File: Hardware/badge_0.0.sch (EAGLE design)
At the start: 48 parts, among them CON1 PH_2, IC1 CP2102, J3 2X6 FEMALE, SW1 MK12C02, SW2 MK12C02, U1 SMBT2222A, U2 SMBT2222A, U4 MCP73832T-2DCI/OT

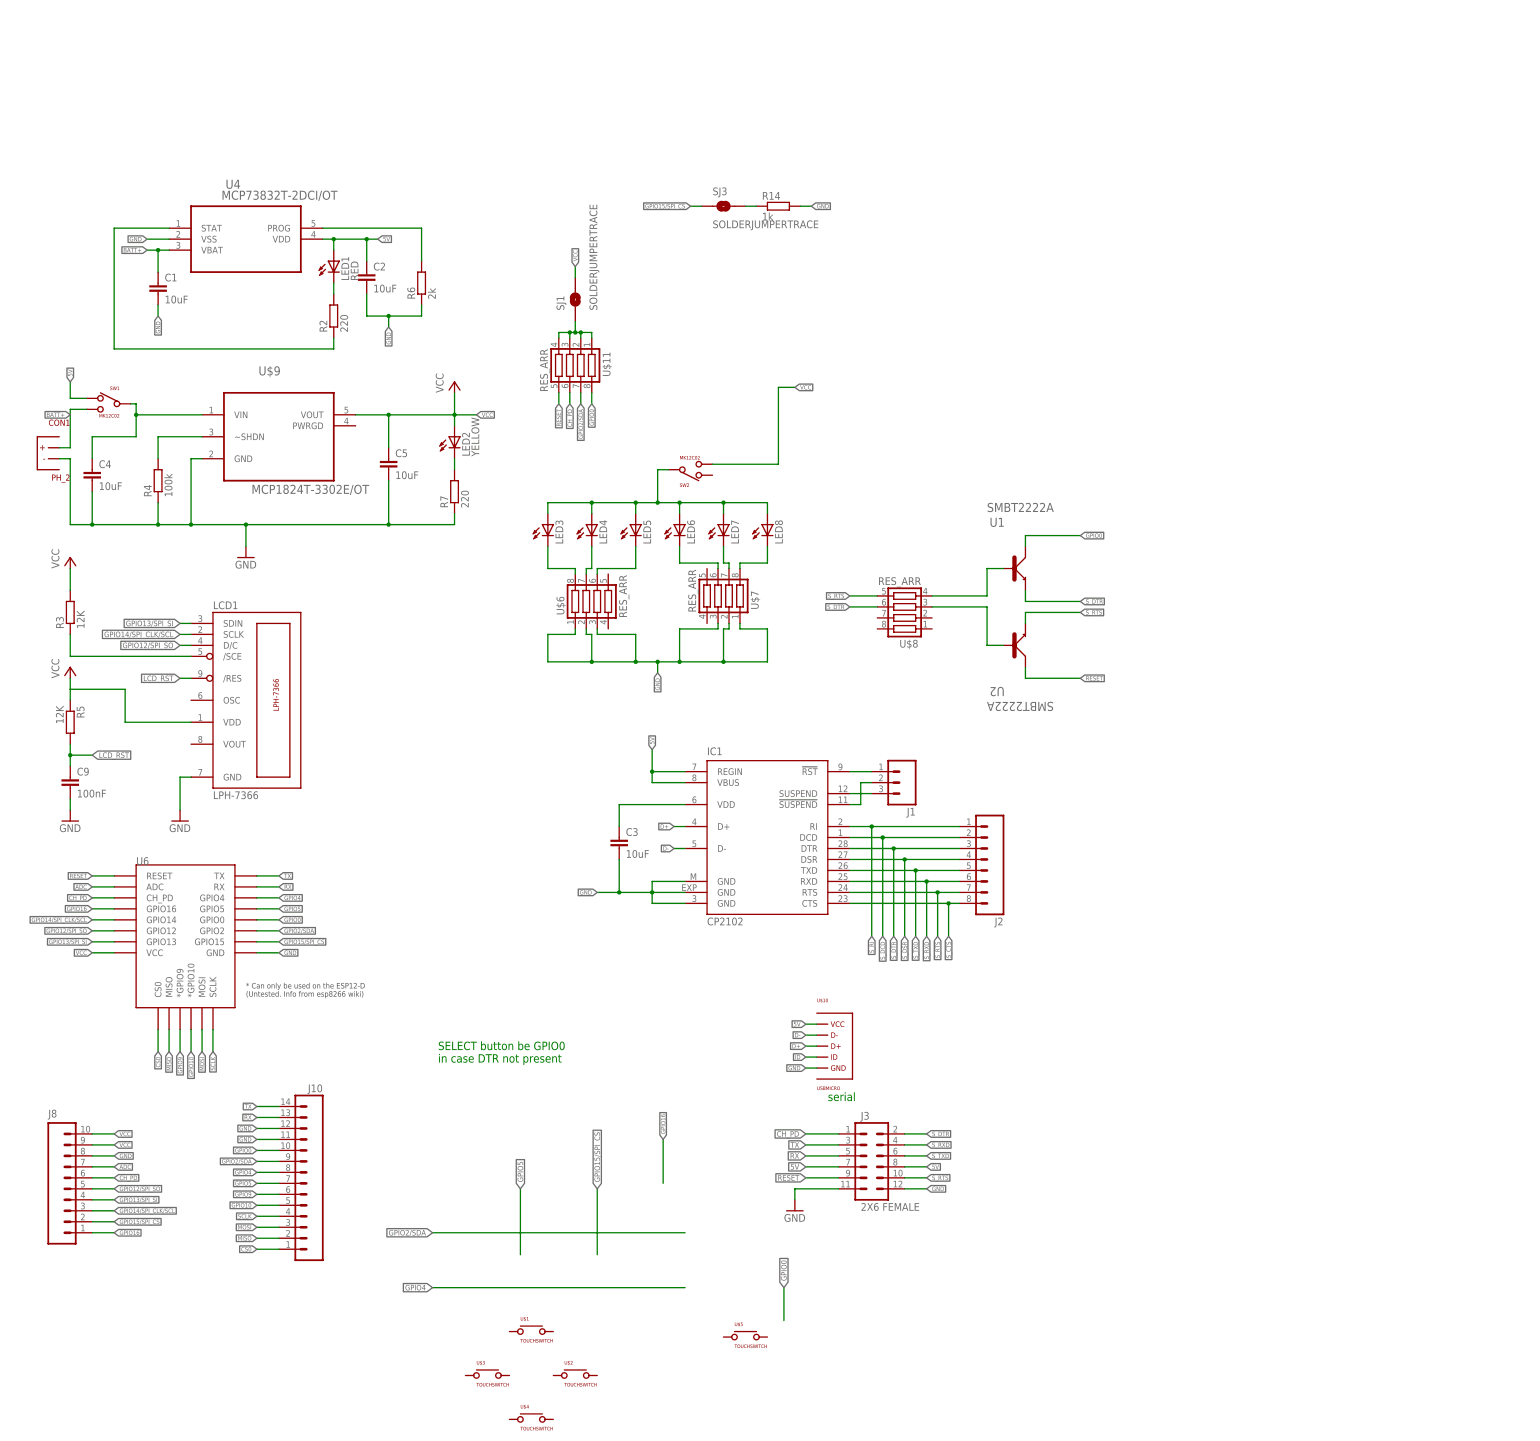
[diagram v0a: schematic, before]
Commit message: Preliminary Neander v0.0
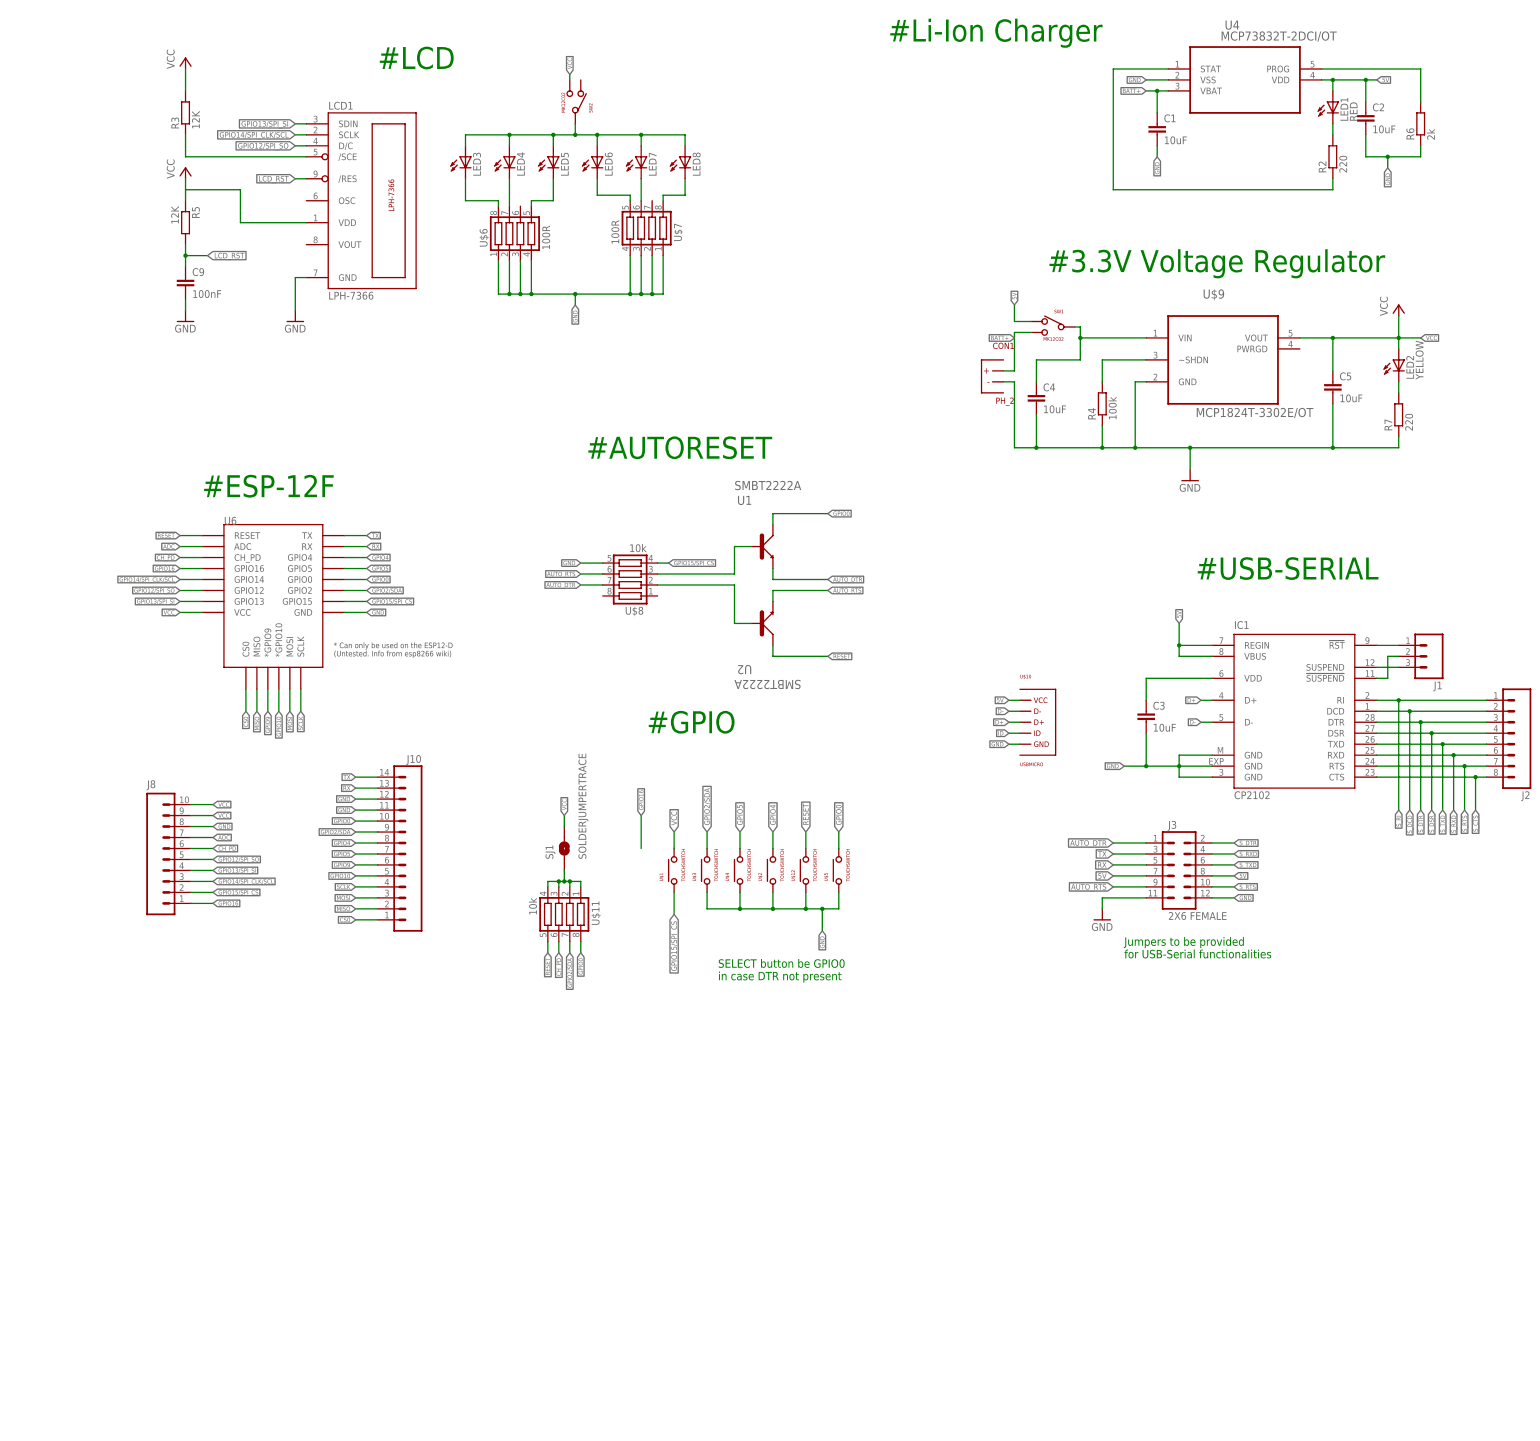
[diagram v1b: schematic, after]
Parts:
- removed R14: 1k, resistor:R-EU_R0603W
- removed SJ3: SOLDERJUMPERTRACE, SparkFun-Retired:SOLDERJUMPERTRACE
- added U$12: TOUCHSWITCH, badge:TOUCHSWITCH
- U$11, U$8: value RES_ARR -> 10k
- U$6, U$7: value RES_ARR -> 100R
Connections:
- removed net N$23: LED7.C, U$7.7
- removed net N$28: R14.1, SJ3.2
- new net AUTO_DTR: J3.1, U$8.7, U1.E
- new net AUTO_RTS: J3.9, U$8.6, U2.E
- new net N$8: LED7.C, U$7.6
- net CH_PD: no longer J3.1
- net GND: now also U$12.P$1, U$2.P$1, U$3.P$1, U$4.P$1, U$5.P$1, U$6.4, U$7.4, U$8.5; no longer R14.2
- net GPIO0: now also U$5.P$2
- net GPIO15/SPI_CS: now also U$1.P$1, U$8.4; no longer SJ3.1
- net GPIO2/SDA: now also U$3.P$2
- net GPIO4: now also U$2.P$2
- net GPIO5: now also U$4.P$2
- net N$13: now also U$6.5; no longer U$6.6
- net N$15: now also U$8.3; no longer U$8.4
- net N$18: now also U$8.2; no longer U$8.3
- net N$22: now also U$7.5; no longer U$7.6
- net RESET: now also U$12.P$2; no longer J3.9
- net S_DTR: no longer U$8.6, U1.E
- net S_RTS: no longer U$8.5, U2.E
- net VCC: now also U$1.P$2
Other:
- note added: "#3.3V Voltage Regulator"
- note added: "#AUTORESET"
- note added: "#ESP-12F"
- note added: "#GPIO"
- note added: "#LCD"
- note added: "#Li-Ion Charger"
- note added: "#USB-SERIAL"
- note added: "Jumpers to be provided for USB-Serial functionalities"
- note removed: "serial"
- moved on the sheet: C1, C2, C3, C4, C5, C9, CON1, IC1, J1, J10, J2, J3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
